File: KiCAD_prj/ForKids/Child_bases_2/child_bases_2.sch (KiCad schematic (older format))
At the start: 61 parts, among them Q1 PN2222A, Q10 PN2222A, Q11 PN2222A, Q2 PN2222A, Q3 PN2222A, Q4 PN2222A, Q5 PN2222A, Q6 2N3904*, Q7 PN2222A, Q8 PN2222A, Q9 PN2222A, SW1 SW_DPST_x2, SW2 SW_DPST_x2, SW3 SW_DPST_x2, SW4 SW_DPST_x2

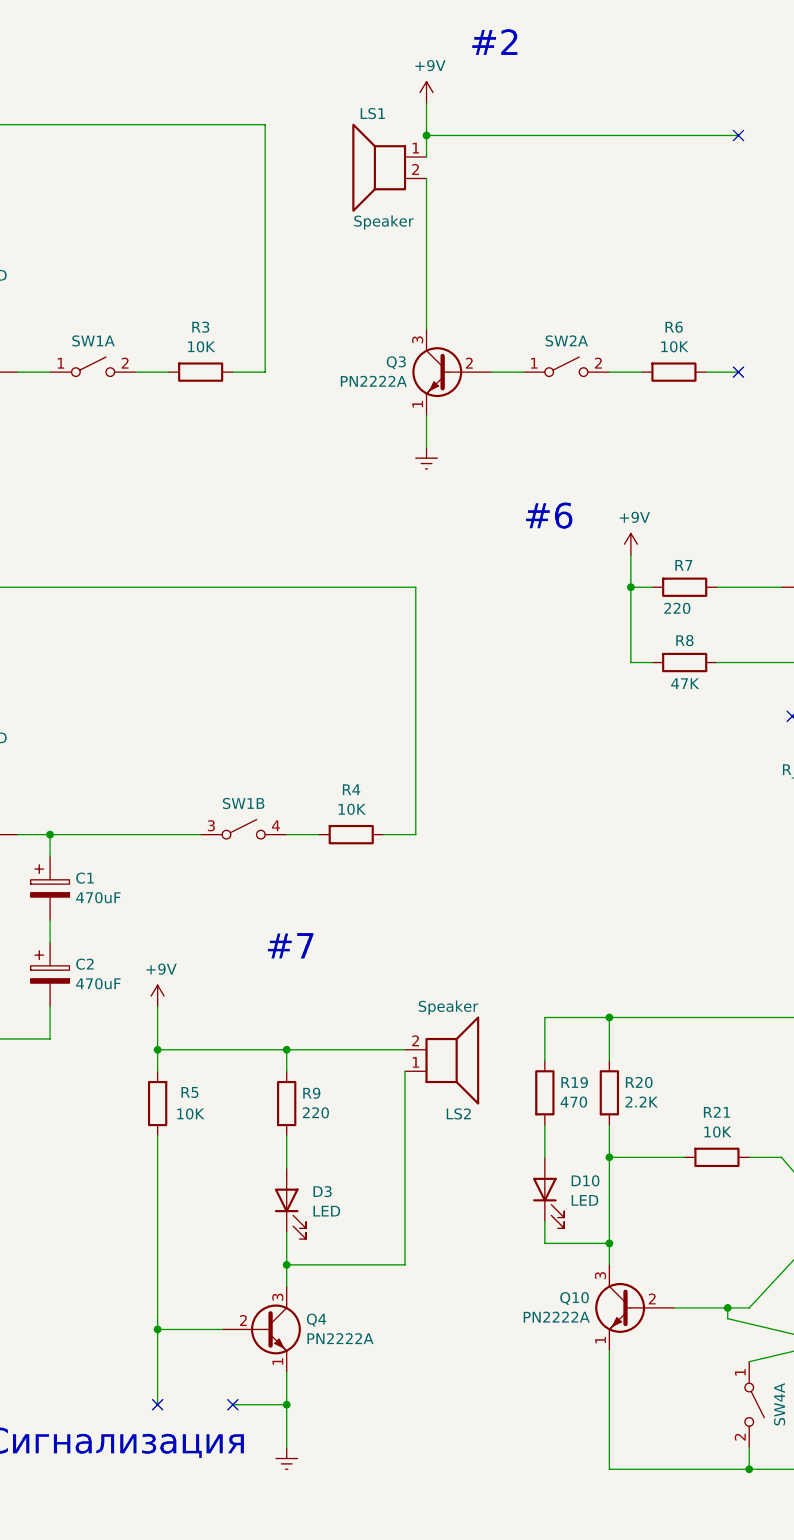
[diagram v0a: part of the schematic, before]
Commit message: Update Child bases2 project
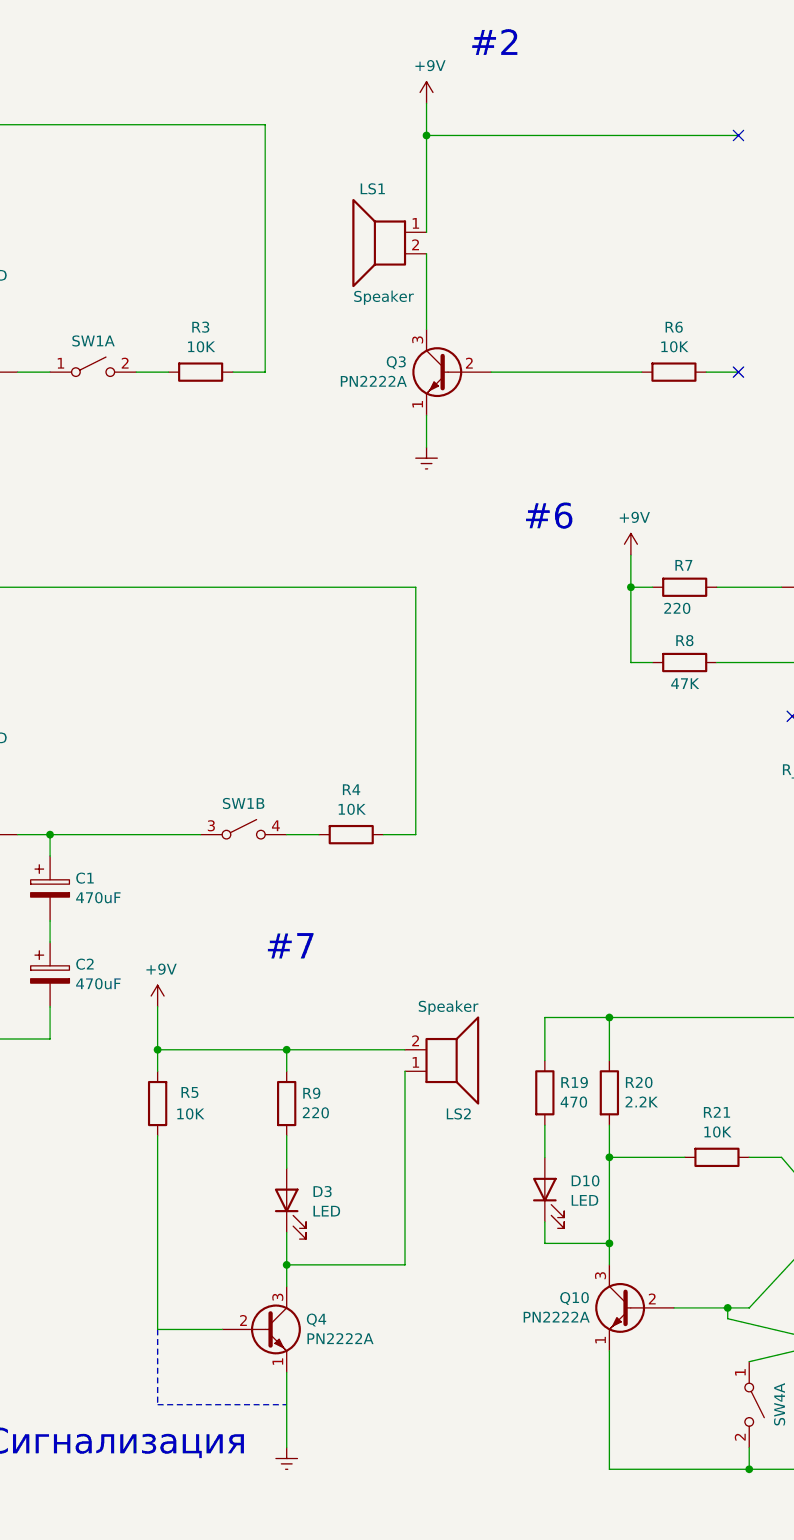
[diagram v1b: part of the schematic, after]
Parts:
- removed unit 1 of SW2
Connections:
- net at Q3.2 (B): now also R6.2
- no-connect marks 5 -> 3
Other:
- moved on the sheet: LS1
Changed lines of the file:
@@
 L Device:Speaker LS1
 U 1 1 5F978E6E
-P 3250 1350
-F 0 "LS1" H 3300 1550 50  0000 C CNN
-F 1 "Speaker" H 3250 1050 50  0000 C CNN
-F 2 "" H 3250 1150 50  0001 C CNN
-F 3 "~" H 3240 1300 50  0001 C CNN
-	1    3250 1350
+P 3250 1700
+F 0 "LS1" H 3300 1900 50  0000 C CNN
+F 1 "Speaker" H 3250 1400 50  0000 C CNN
+F 2 "" H 3250 1500 50  0001 C CNN
+F 3 "~" H 3240 1650 50  0001 C CNN
+	1    3250 1700
 	-1   0    0    -1
-$EndComp
-$Comp
-L Switch:SW_DPST_x2 SW2
-U 1 1 5F97A5C2
-P 4100 2350
-F 0 "SW2" H 4100 2493 50  0000 C CNN
-F 1 "SW_DPST_x2" H 4100 2494 50  0001 C CNN
-F 2 "" H 4100 2350 50  0001 C CNN
-F 3 "~" H 4100 2350 50  0001 C CNN
-	1    4100 2350
-	1    0    0    -1
 $EndComp
 $Comp
@@
 	3450 2700 3450 2550
 Wire Wire Line
-	3750 2350 3900 2350
-Wire Wire Line
-	4300 2350 4450 2350
-Wire Wire Line
 	4900 2350 4750 2350
-Wire Wire Line
-	3450 1450 3450 2150
 $Comp
 L power:+9V #PWR05
@@
 	1    0    0    -1
 $EndComp
-Wire Wire Line
-	2800 7000 2800 7150
-Wire Wire Line
-	2200 6800 2200 7150
-Connection ~ 2200 6800
-NoConn ~ 2200 7150
-Wire Wire Line
-	2800 7150 2550 7150
-Connection ~ 2800 7150
-Wire Wire Line
-	2800 7150 2800 7350
-NoConn ~ 2550 7150
 Text Notes 850  900  0    118  ~ 0
 #1
@@
 	3450 1250 4900 1250
 Connection ~ 3450 1250
-Wire Wire Line
-	3450 1250 3450 1350
 NoConn ~ 4900 1250
 $Comp
@@
 Wire Wire Line
 	5950 6700 5800 6700
+Wire Wire Line
+	3750 2350 4450 2350
+Wire Wire Line
+	3450 1250 3450 1700
+Wire Wire Line
+	3450 1800 3450 2150
+Wire Wire Line
+	2800 7000 2800 7350
+Wire Notes Line
+	2200 6800 2200 7150
+Wire Notes Line
+	2200 7150 2800 7150
 $EndSCHEMATC
